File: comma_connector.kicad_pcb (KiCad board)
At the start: 2 copper layers, 60 x 80.5 mm, 2 parts, among them J1 2317507-1, J2 Screw_Terminal_01x12

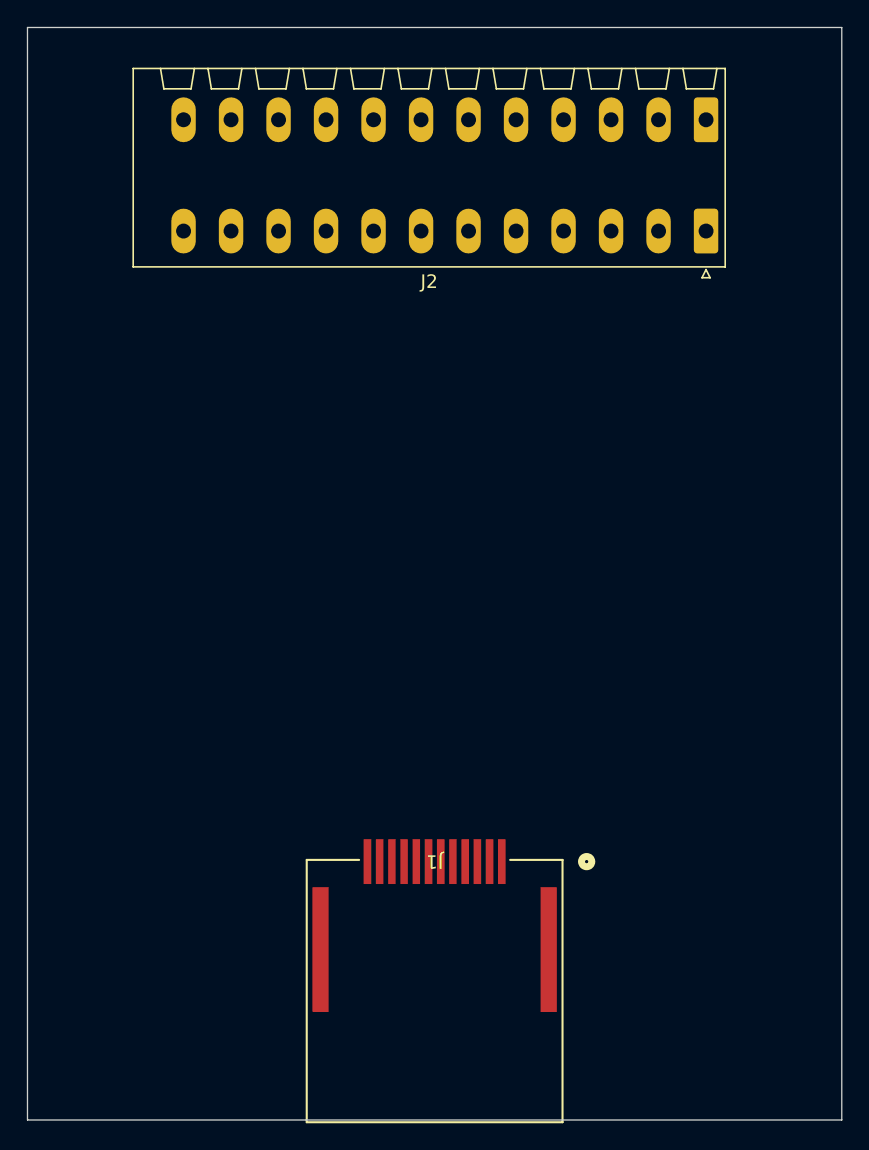
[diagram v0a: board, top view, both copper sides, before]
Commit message: align and finish trace routes
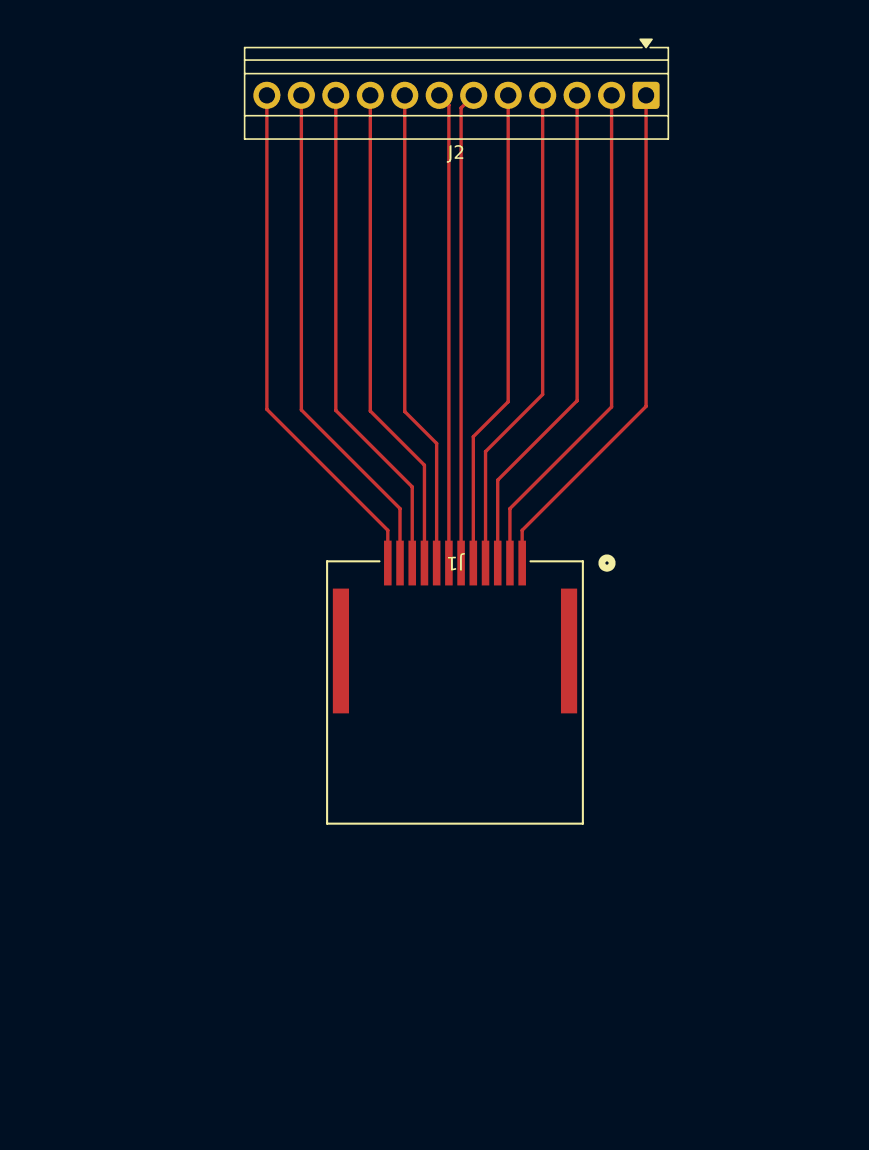
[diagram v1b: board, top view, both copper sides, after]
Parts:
- J2: footprint Connector_Phoenix_SPT:PhoenixContact_SPT_1.5_12-H-3.5_1x12_P3.5mm_Horizontal -> TerminalBlock:TerminalBlock_Xinya_XY308-2.54-12P_1x12_P2.54mm_Horizontal
- moved J1 22.1 mm to (201.5, 104.0)
- moved J2 10.9 mm to (215.6, 60.0)
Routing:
- net Net-(J2-Pin_1): track 0.00 -> 38.2 mm
- net Net-(J2-Pin_12): track 0.00 -> 38.2 mm
- net Net-(J2-Pin_2): track 0.00 -> 37.6 mm
- net Net-(J2-Pin_11): track 0.00 -> 37.5 mm
- net Net-(J2-Pin_3): track 0.00 -> 36.9 mm
- net Net-(J2-Pin_10): track 0.00 -> 36.8 mm
- net Net-(J2-Pin_4): track 0.00 -> 36.2 mm
- net Net-(J2-Pin_5): track 0.00 -> 35.5 mm
- net Net-(J2-Pin_6): track 0.00 -> 35.4 mm
- net Net-(J2-Pin_8): track 0.00 -> 35.4 mm
- net Net-(J2-Pin_9): track 1.00 -> 36.1 mm
- net Net-(J2-Pin_7): track 0.08 -> 34.8 mm
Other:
- board outline removed
